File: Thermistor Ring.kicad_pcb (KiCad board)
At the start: 2 copper layers, 48.3 x 48.3 mm, 18 parts, among them J1 Conn_01x04_Socket, U1 TPS7A2018PDBVR, U2 MCP9808T-E/MC, U3 MCP9808T-E/MC, U4 MCP9808T-E/MC, U5 MCP9808T-E/MC, U6 MCP9808T-E/MC, U7 MCP9808T-E/MC

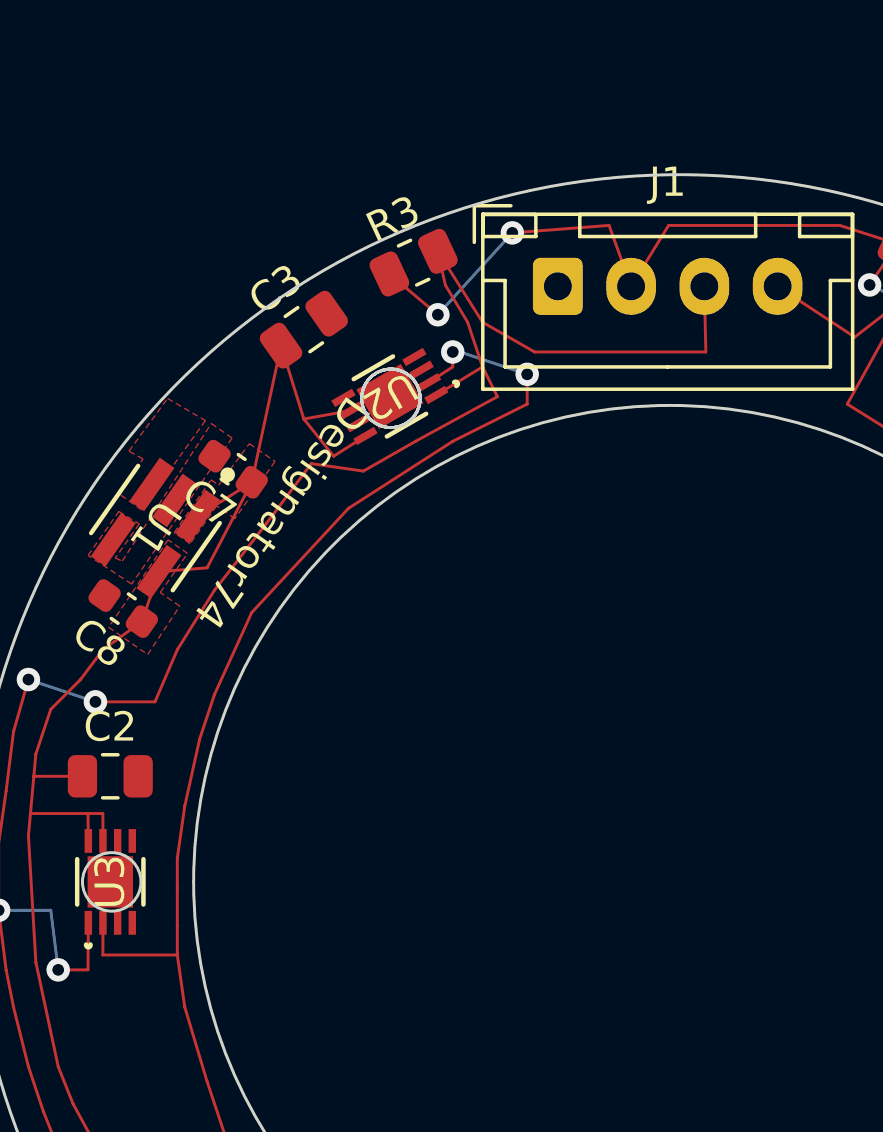
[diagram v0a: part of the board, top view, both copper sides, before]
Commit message: wip: some fixes
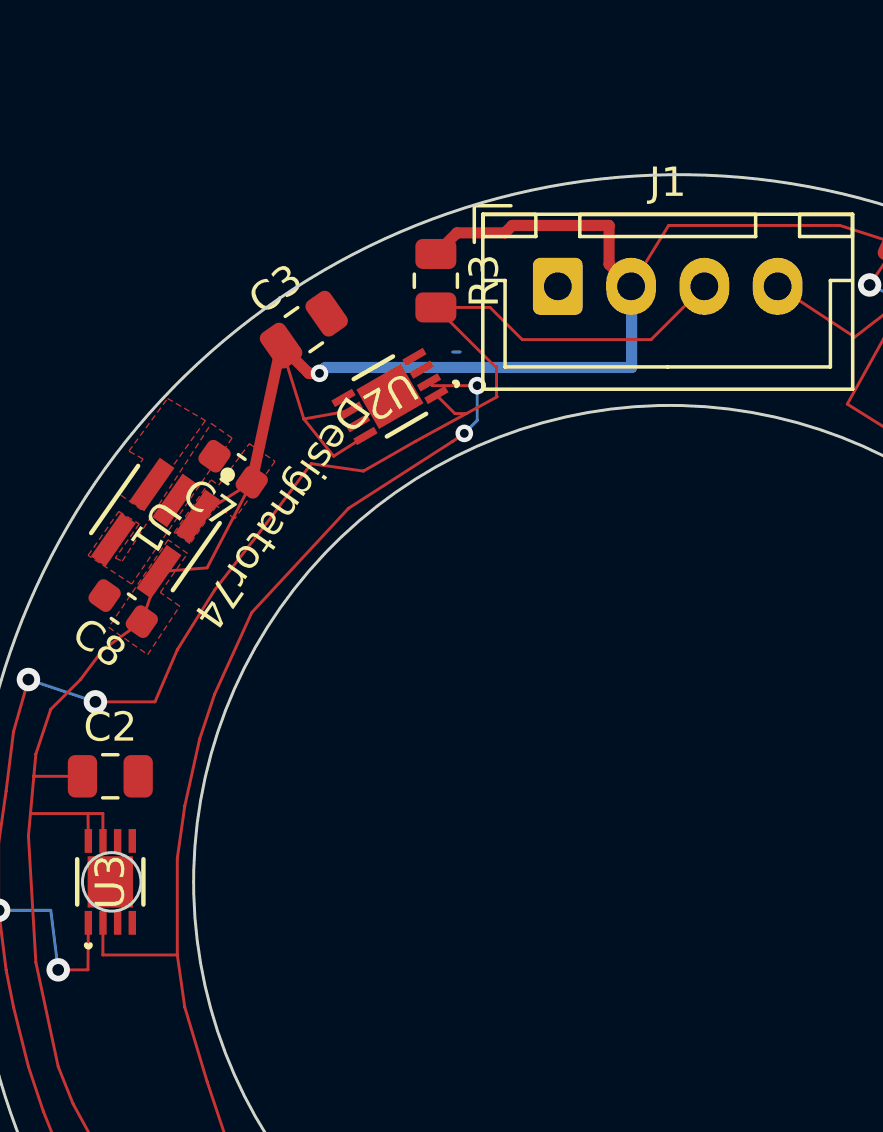
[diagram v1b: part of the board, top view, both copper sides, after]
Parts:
- moved R3 0.98 mm to (66.5, 35.2), turned to -90 degrees
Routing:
- net /Power 3.3-5V: track 179.9 -> 192.3 mm, vias 4 -> 3
- net /SDA: track 175.9 -> 171.3 mm
- net /SCL: track 132.0 -> 128.0 mm
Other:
- outline, holes or cut-outs redrawn
